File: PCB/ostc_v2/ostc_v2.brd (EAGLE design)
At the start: 31.5 x 54.8 mm, 13 parts, among them U1 ICO-640-SGG, U2 XC9536XL-10CSG48I, U3 IS62C256AL-45TLI, U4 LP5912Q3.3DRVRQ1, X1 5055670651, X2 5055670251, X3 150-10-640-00-001000

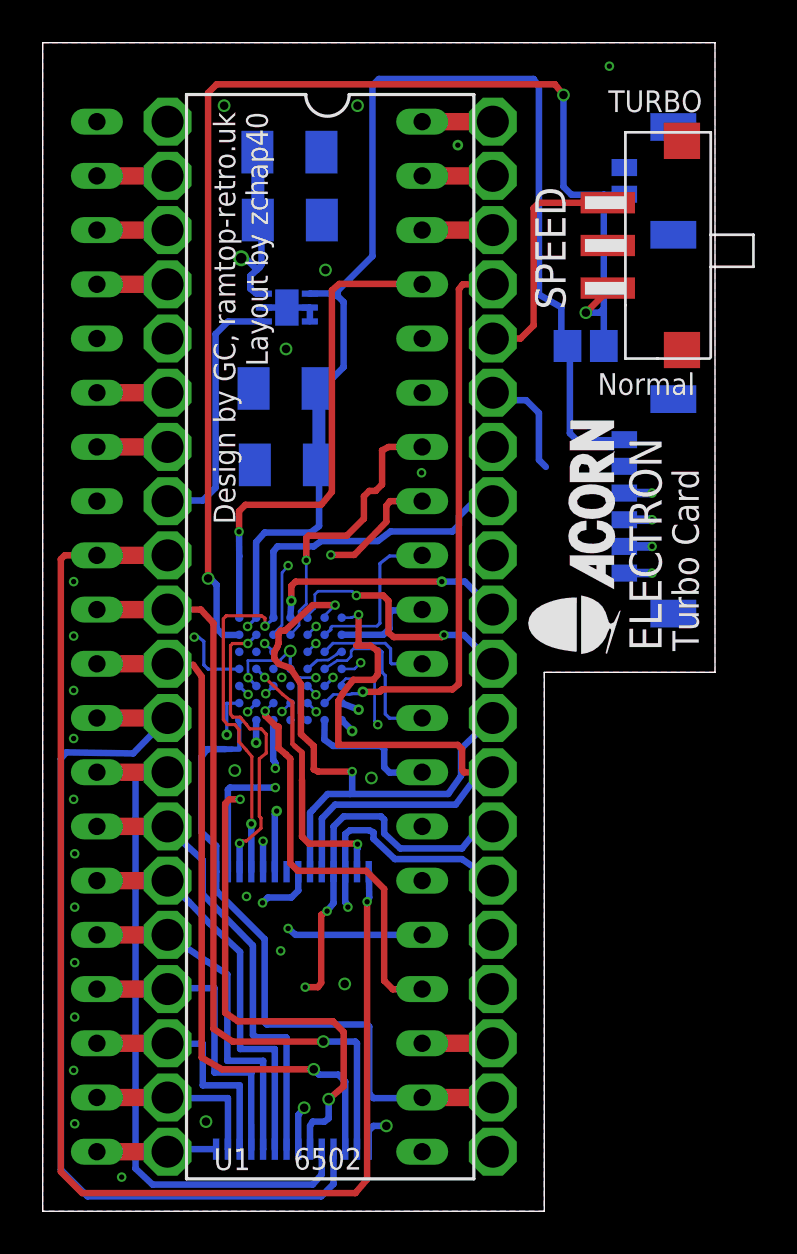
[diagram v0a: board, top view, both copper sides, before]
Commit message: Updated PCBs, schematics, gerbers & renders
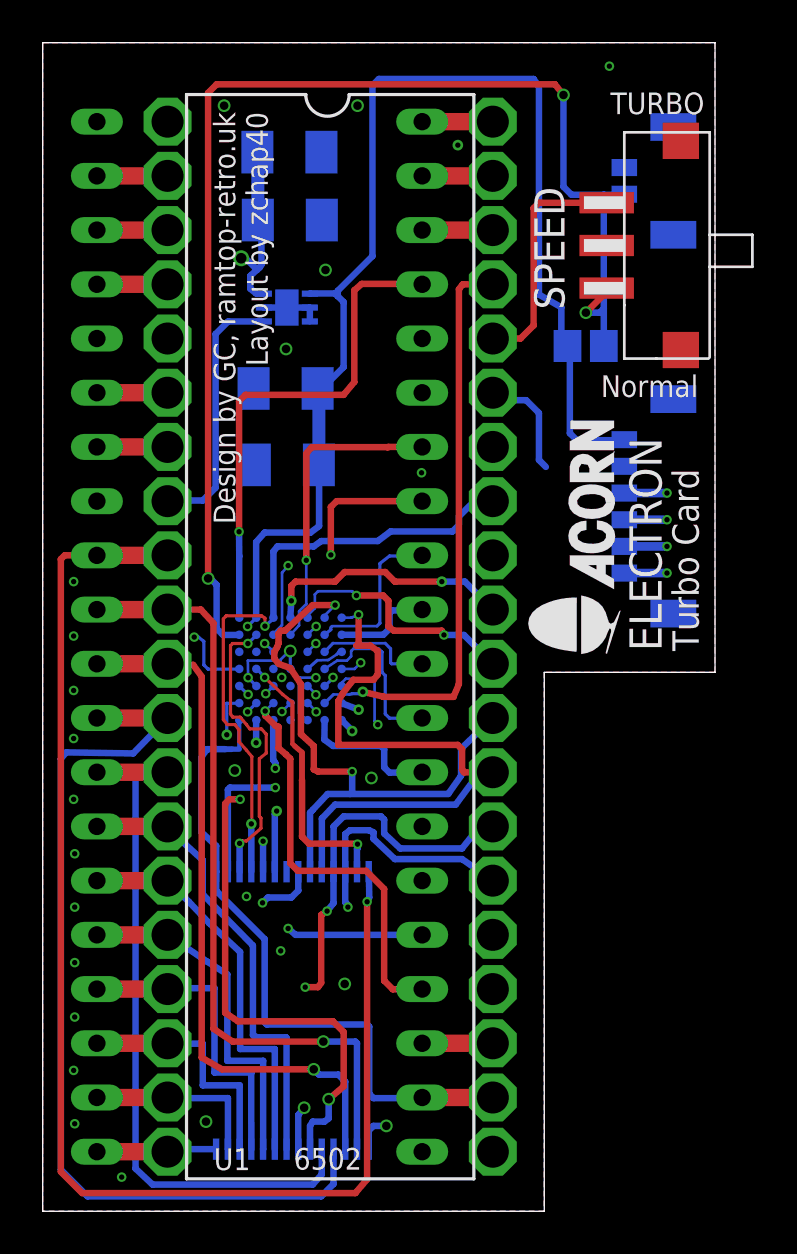
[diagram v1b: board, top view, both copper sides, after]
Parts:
- moved S1 0.05 mm to (27.9, 45.2)
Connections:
- net GND: now also S1.P$1, S1.P$2
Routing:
- net N$55: track 66.7 -> 68.1 mm
- net N$56: track 65.5 -> 66.9 mm
- net N$58: track 67.8 -> 69.2 mm
- net N$57: track 76.3 -> 77.7 mm
- net N$30: track 13.6 -> 14.4 mm
- net N$29: track 10.0 -> 10.9 mm
